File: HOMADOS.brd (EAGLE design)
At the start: 83.5 x 78.7 mm, 72 parts, among them P1 39-30-02?, P10 39-30-02?, P11 39-30-02?, P12 39-30-02?, P13 39-30-02?, P14 39-30-02?, P15 39-30-02?, P16 39-30-02?, P17 39-30-02?, P2 39-30-02?, P3 39-30-02?, P4 39-30-02?, P5 39-30-02?, P6 39-30-02?, P7 39-30-02?, P8 39-30-02?, P9 39-30-02?, Q1 T460, Q10 T460, Q11 T460, Q12 T460, Q13 T460, Q14 T460, Q15 T460, Q16 T460, Q2 T460, Q3 T460, Q4 T460, Q5 T460, Q6 T460, Q7 T460, Q8 T460, Q9 T460, U1 ARDUINO-MEGA-SOLINOID

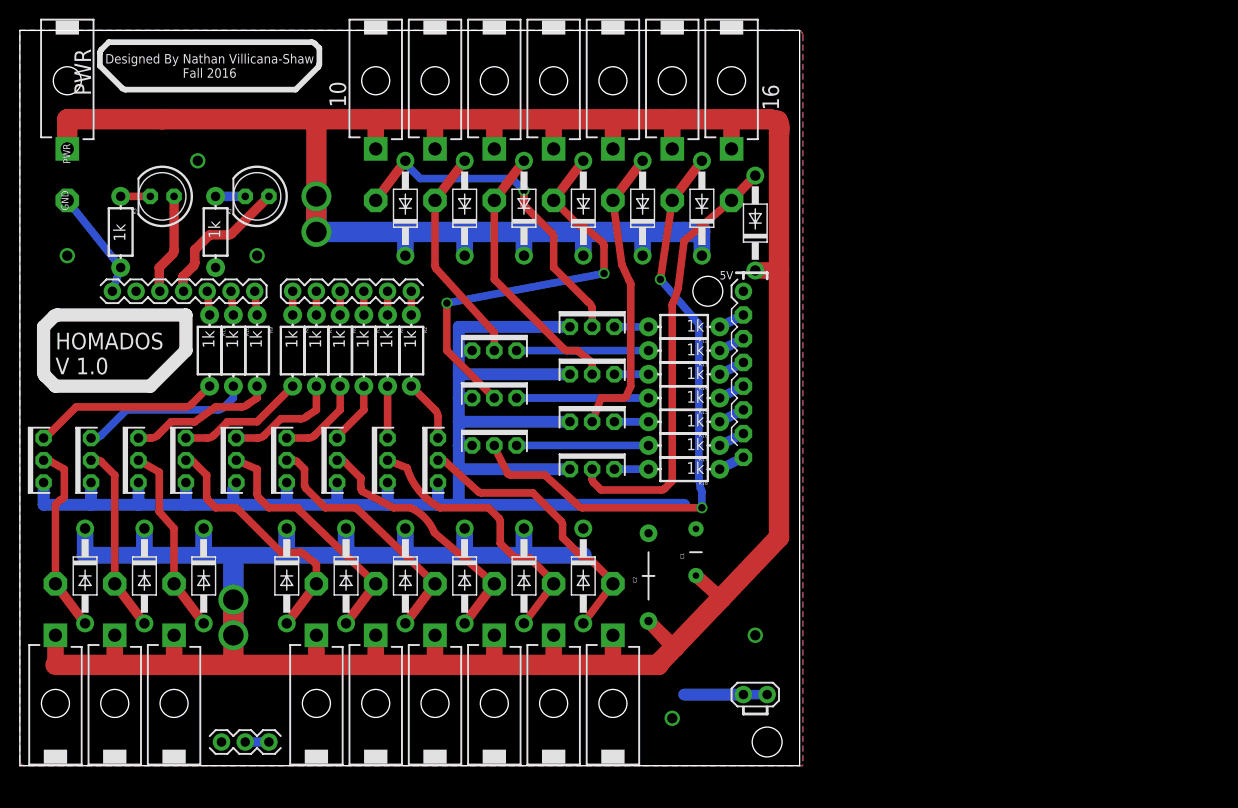
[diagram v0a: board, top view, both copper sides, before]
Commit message: created v2 of Homados board
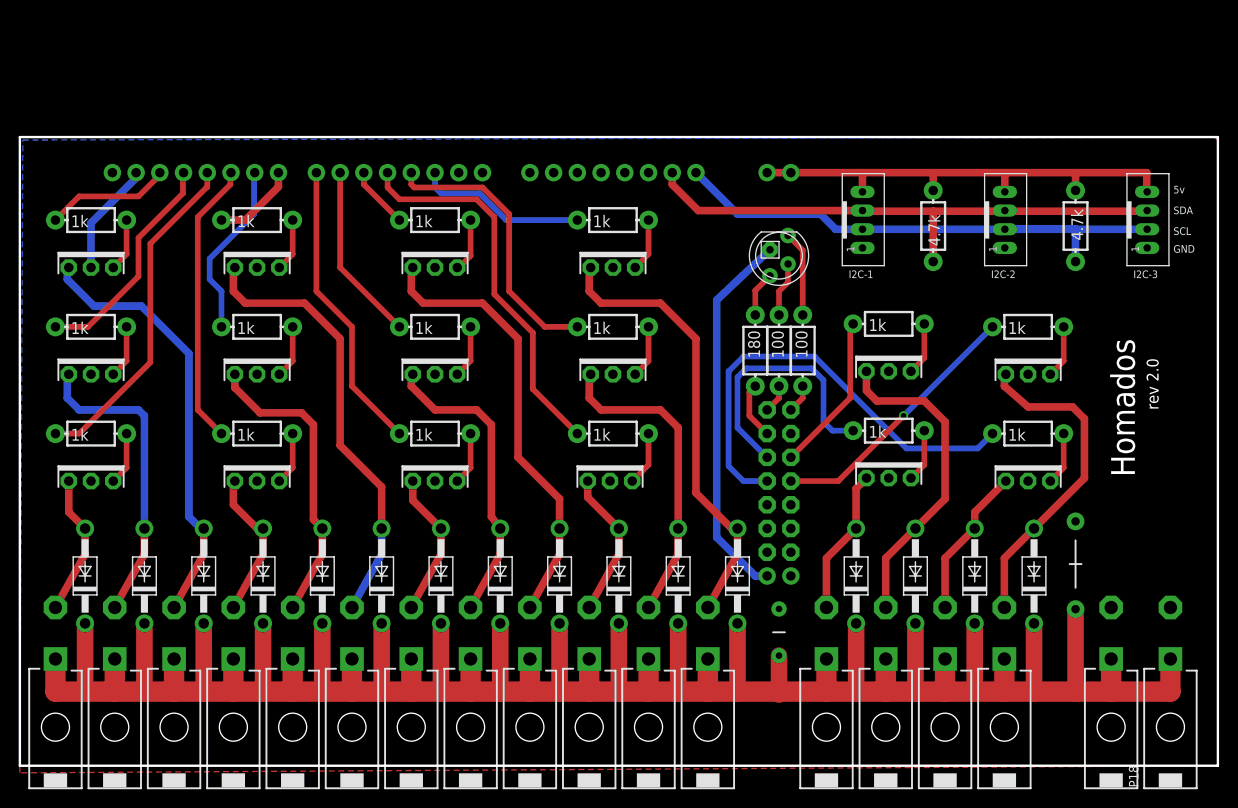
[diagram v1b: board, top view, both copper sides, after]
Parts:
- removed LED1, LED2: (no value), adafruit:LED5MM
- removed U1: ARDUINO-MEGA-SOLINOID, Nathans-Arduinos2:ARDUINO_MEGA-SOLINOID
- added I2C-1, I2C-2, I2C-3: JST-PH_4-PIN_HEADER, JST_connectors:JST_B4B-PH_HEADER
- added P18: 39-30-02?, con-molex-mini-fit:39-30-?02?
- added R19: 1k, SparkFun-Passives:AXIAL-0.3-KIT
- added R20, R21: 100, SparkFun-Passives:AXIAL-0.3-KIT
- added U$2: RGBLED_CA, adafruit:LED5MMRGB
- added U2: ARDUINO-MEGAPRO-5V, SparkFun-Minimal-Shields:ARDUINO_MEGA-PRO-5V
- R1, R2: value 1k -> 4.7k
- R3: value 1k -> 180
- moved P2 124.4 mm to (116.8, 11.4), turned to 0 degrees
- moved R1 76.8 mm to (97.8, 57.8), turned to 90 degrees
- moved P14 72.9 mm to (105.4, 11.4), turned to 0 degrees
- moved R2 72.4 mm to (113.0, 57.8)
- moved R3 69.1 mm to (78.7, 44.5)
- moved P15 65.2 mm to (99.1, 11.4), turned to 0 degrees
- moved Q9 64.4 mm to (63.5, 53.3), turned to 0 degrees
- moved D13 62.3 mm to (108.6, 20.3)
- moved P11 59.2 mm to (61.0, 11.4), turned to 0 degrees
- moved P12 59.2 mm to (67.3, 11.4), turned to 0 degrees
- moved P13 59.2 mm to (73.7, 11.4), turned to 0 degrees
- moved P16 59.2 mm to (92.7, 11.4), turned to 0 degrees
- moved Q15 57.3 mm to (108.0, 30.5)
- moved P17 55.5 mm to (86.4, 11.4), turned to 0 degrees
- moved Q12 54.9 mm to (7.62, 30.5)
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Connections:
- removed net D10: R17.P$1, U1.32
- removed net D12: R18.P$1, U1.34
- removed net D2: R13.P$1, U1.24
- removed net D4: R14.P$1, U1.26
- removed net D6: R15.P$1, U1.28
- removed net D8: R16.P$1, U1.30
- removed net N$5: U1.13
- new net 5V: I2C-1.P4, I2C-2.P4, I2C-3.P4, R1.P$2, R2.P$1, U2.5V@1, U2.5V@2
- new net A0: R3.P$1, U$2.4
- new net A2: R20.P$1, U$2.1
- new net ARDUINO_GND: U$2.2, U2.GND@2
- new net BLUE: R3.P$2, U2.42
- new net GREEN: R21.P$2, U2.22
- new net N$12: U2.18
- new net N$13: U2.19
- new net N$17: U2.43
- new net N$28: U2.48
- new net N$29: U2.49
- new net N$32: U2.50
- new net N$6: Q1.3, R19.P$2
- new net N$8: U2.16
- new net N$9: U2.17
- new net N23: U2.51
- new net N24: U2.52
- new net N25: U2.53
- new net PW11: R9.P$1, U2.13
- new net PW12: R18.P$1, U2.44
- new net PW13: R17.P$1, U2.45
- new net PW14: R16.P$1, U2.46
- new net RED: R20.P$2, U2.23
- new net SCL: I2C-1.P2, I2C-2.P2, I2C-3.P2, R2.P$2, U2.21
- new net SDA: I2C-1.P3, I2C-2.P3, I2C-3.P3, R1.P$1, U2.20
- net D0: now also R15.P$1, U2.47; no longer R12.P$1, U1.22
- net GND: now also I2C-1.P1, I2C-2.P1, I2C-3.P1, P18.2, Q1.2, Q10.2, Q11.2, Q12.2, Q13.2, Q14.2, Q15.2, Q16.2, Q2.2, Q3.2, Q4.2, Q5.2, Q6.2, Q7.2, Q8.2, Q9.2, U2.GND@3, U2.GND@4; no longer Q1.1, Q10.1, Q11.1, Q12.1, Q13.1, Q14.1, Q15.1, Q16.1, Q2.1, Q3.1, Q4.1, Q5.1, Q6.1, Q7.1, Q8.1, Q9.1, R1.P$2, R3.P$2, U1.GND@0, U1.GND@1, U1.GND@2, U1.GND@3, U1.GND@4
- net N$1: now also R21.P$1, U$2.3; no longer LED1.K, R1.P$1
- net N$11: now also Q3.1; no longer Q3.2
- net N$15: now also Q4.1; no longer Q4.2
- net N$19: now also Q8.1; no longer Q5.2
- net N$2: now also Q1.1; no longer Q1.2
- net N$22: now also Q8.3; no longer Q5.3
- net N$23: now also Q7.1; no longer Q6.2
- net N$26: now also Q7.3; no longer Q6.3
- net N$27: now also Q6.1; no longer Q7.2
- net N$3: now also U2.14; no longer LED2.K, R3.P$1
- net N$30: now also Q6.3; no longer Q7.3
- net N$31: now also Q5.1; no longer Q8.2
- net N$34: now also Q5.3; no longer Q8.3
- net N$35: now also Q12.1; no longer Q9.2
- net N$38: now also Q12.3; no longer Q9.3
- net N$39: now also Q11.1; no longer Q10.2
- net N$4: now also Q2.1; no longer Q2.2
- net N$42: now also Q11.3; no longer Q10.3
- net N$43: now also Q10.1; no longer Q11.2
- net N$46: now also Q10.3; no longer Q11.3
- net N$47: now also Q9.1; no longer Q12.2
- net N$50: now also Q9.3; no longer Q12.3
- net N$51: now also Q16.1; no longer Q13.2
- net N$54: now also Q16.3; no longer Q13.3
- net N$55: now also Q15.1; no longer Q14.2
- net N$58: now also Q15.3; no longer Q14.3
- net N$59: now also Q14.1; no longer Q15.2
- net N$62: now also Q14.3; no longer Q15.3
- net N$63: now also Q13.1; no longer Q16.2
- net N$66: now also Q13.3; no longer Q16.3
- net N$7: now also U2.15; no longer Q1.3, R2.P$2
- net PW0: now also R14.P$1, U2.2; no longer R2.P$1, U1.2
- net PW1: now also R13.P$1, U2.3; no longer R4.P$1, U1.3
- net PW10: now also R10.P$1, U2.12; no longer LED2.A, U1.12
- net PW2: now also R12.P$1, U2.4; no longer R5.P$1, U1.4
- net PW3: now also R19.P$1, U2.5; no longer R6.P$1, U1.5
- net PW4: now also R4.P$1, U2.6; no longer R7.P$1, U1.6
- net PW5: now also R5.P$1, U2.7; no longer R8.P$1, U1.7
- net PW6: now also R6.P$1, U2.8; no longer R9.P$1, U1.8
- net PW7: now also R7.P$1, U2.9; no longer R10.P$1, U1.9
- net PW8: now also R8.P$1, U2.10; no longer R11.P$1, U1.10
- net PW9: now also R11.P$1, U2.11; no longer LED1.A, U1.11
- net PWR: now also P18.1
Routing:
- net PWR: track 494.9 -> 312.1 mm, vias 4 -> 0
- net GND: track 184.3 -> 12.2 mm, vias 5 -> 0
- net SCL: track 0.00 -> 61.9 mm
- net SDA: track 0.00 -> 59.9 mm
- net 5V: track 0.00 -> 50.7 mm
- net PW14: track 0.00 -> 48.6 mm
- net ARDUINO_GND: track 0.00 -> 40.4 mm
- net PW2: track 2.54 -> 41.2 mm
- net N$63: track 46.8 -> 15.6 mm
- net N$59: track 65.3 -> 34.4 mm, vias 2 -> 0
- net PW5: track 2.54 -> 31.6 mm
- net PW12: track 0.00 -> 28.0 mm
- net PW8: track 2.55 -> 30.5 mm
- net PW1: track 2.54 -> 30.2 mm
- net N$27: track 20.4 -> 46.5 mm
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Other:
- board size 83.5 x 78.7 mm -> 128.3 x 67.3 mm
- board text added: "5v"
- board text added: "Homados"
- board text added: "SCL"
- board text added: "SDA"
- board text added: "rev 2.0"
- board text removed: "10"
- board text removed: "16"
- board text removed: "Designed By Nathan Villicana-Shaw Fall 2016"
- board text removed: "HOMADOS V 1.0"
- board text removed: "PWR"
